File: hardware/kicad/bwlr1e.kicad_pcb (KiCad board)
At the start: 2 copper layers, 36.8 x 90.9 mm, 68 parts, among them Q1 AO3407, Q2 DMG1012UW, SW3 RESET, SW4 BOOT, U1 BME680, U2 RAK3172, U3 AEM10941-QFN, U4 XC6215

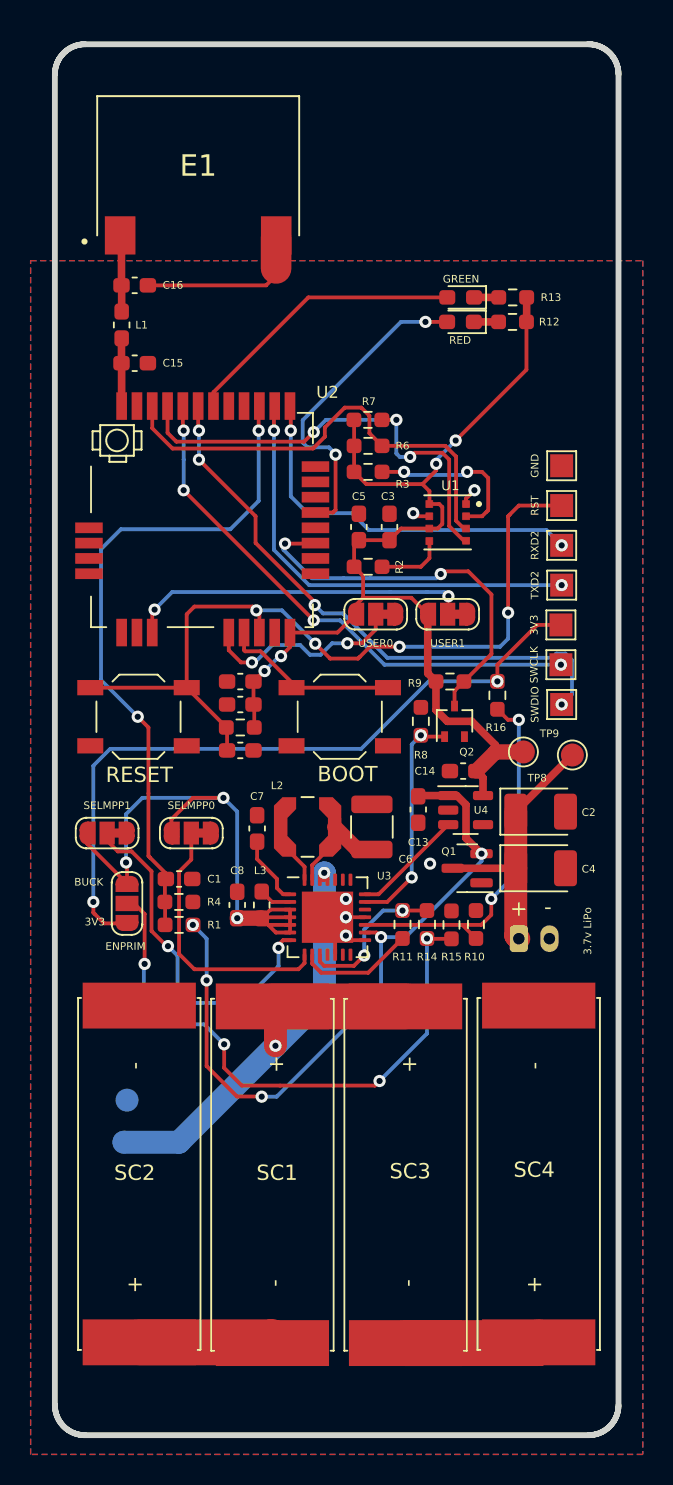
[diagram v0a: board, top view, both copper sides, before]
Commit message: revision 2
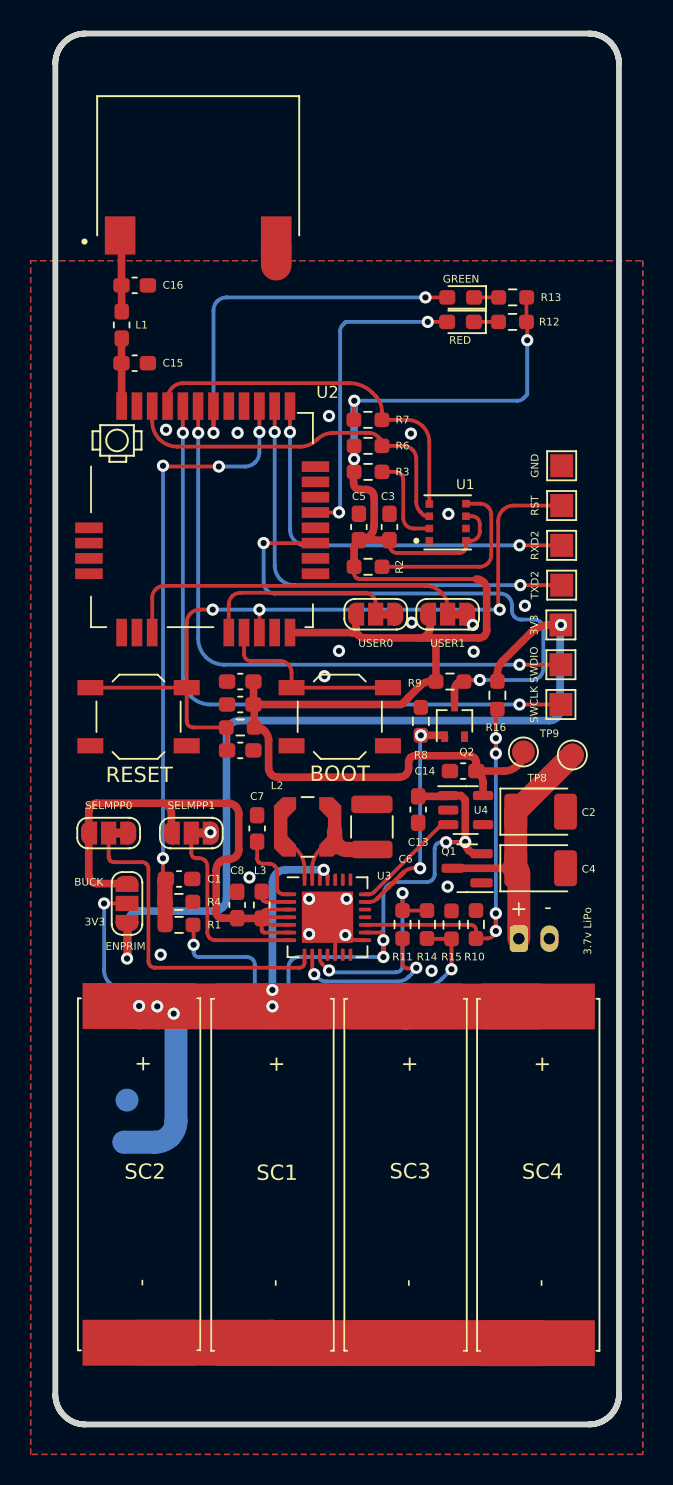
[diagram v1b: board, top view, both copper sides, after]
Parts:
- moved JP4 5.50 mm to (137.0, 105.4)
- moved JP3 5.40 mm to (131.6, 105.4)
- moved TP3 2.60 mm to (161.2, 94.4)
- moved TP6 2.60 mm to (161.2, 97.0)
- moved REF** 0.70 mm to (149.8, 96.0)
- moved SC2 0.59 mm to (133.9, 127.7), turned to -90 degrees
- moved SC4 0.57 mm to (160.0, 127.7), turned to -90 degrees
- turned U1 to 180 degrees
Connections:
- SC1 pad 2: Net-(SC1-Pad2) -> GND
- SC2 pad 1: Net-(SC1-Pad2) -> /SOLAR+
- SC3 pad 2: Net-(SC3-Pad2) -> GND
- SC4 pad 1: Net-(SC3-Pad2) -> /SOLAR+
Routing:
- net +3V3: track 71.9 -> 115.6 mm, vias 4 -> 3
- net /SOLAR+: track 37.5 -> 53.1 mm, vias 2 -> 6
- net GND: track 21.2 -> 32.3 mm, vias 6 -> 20
- net Net-(Q2-Pad3): track 25.9 -> 36.3 mm
- net /SELMPP1: track 23.0 -> 12.9 mm, vias 2 -> 0
- net /EXT_3V3: track 47.1 -> 57.1 mm
- net Net-(SC1-Pad2): track 8.72 -> 0.00 mm
- net Net-(SC3-Pad2): track 8.72 -> 0.00 mm
- net /SWCLK: track 34.9 -> 43.4 mm, vias 4 -> 2
- net Net-(R2-Pad2): track 4.47 -> 12.3 mm
- net /LED2: track 18.7 -> 25.5 mm, vias 0 -> 2
- net /SDA: track 30.5 -> 24.5 mm
- net /SCL: track 30.5 -> 24.5 mm, vias 3 -> 0
- net Net-(R3-Pad2): track 11.0 -> 6.26 mm, vias 2 -> 0
- net /BATT_MEAS: track 44.2 -> 39.9 mm, vias 2 -> 4
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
